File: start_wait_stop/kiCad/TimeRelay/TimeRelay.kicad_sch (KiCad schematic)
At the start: 15 parts, among them J1 230V AC Input, J10 Relay, J2 230V AC Input, J3 Relay, J4 Relay, J5 230V AC OUTPUT, J6 230V AC OUTPUT, J7 Relay, J8 Relay, J9 Relay, K1 FINDER-32.21-x000, SW1 Start

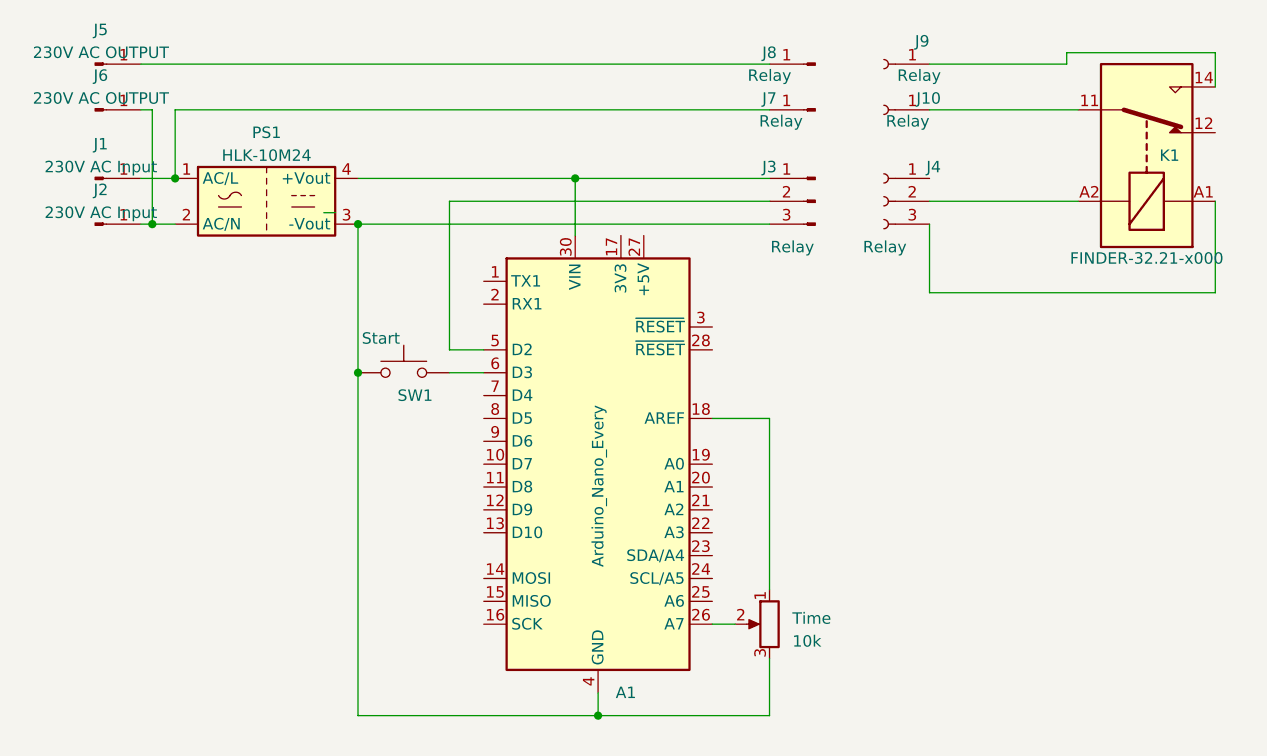
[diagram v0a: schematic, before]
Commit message: Playing arround witj KiCAD.
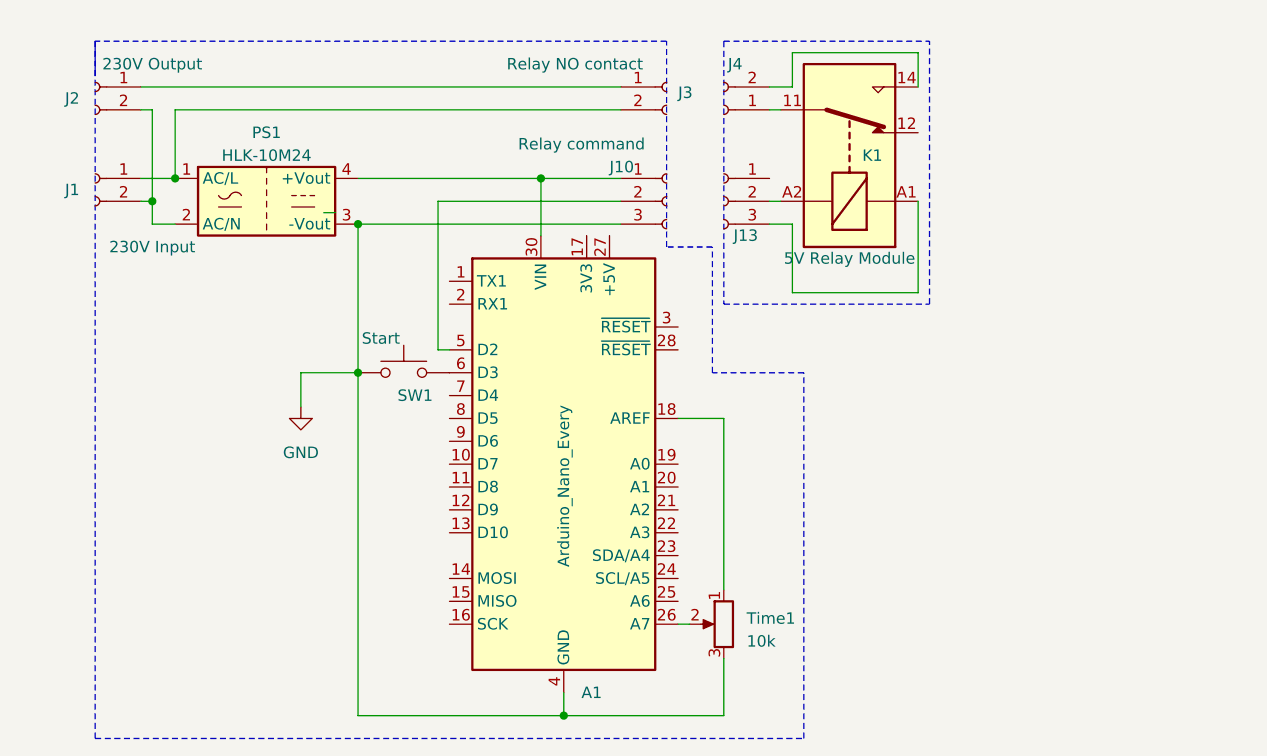
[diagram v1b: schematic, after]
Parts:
- removed J1, J2: 230V AC Input, symbol Connector:Conn_01x01_Pin
- removed J10, J9: Relay, symbol Connector:Conn_01x01_Socket
- removed J3: Relay, symbol Connector:Conn_01x03_Pin
- removed J4: Relay, symbol Connector:Conn_01x03_Socket
- removed J5, J6: 230V AC OUTPUT, symbol Connector:Conn_01x01_Pin
- removed J7, J8: Relay, symbol Connector:Conn_01x01_Pin
- added J1: 230V Input, Connector_Wire:SolderWire-1.5sqmm_1x02_P7.8mm_D1.7mm_OD3.9mm, symbol Connector:Conn_01x02_Socket
- added J10: Relay command, Connector_PinSocket_2.54mm:PinSocket_1x03_P2.54mm_Vertical, symbol Connector:Conn_01x03_Socket
- added J13: Relay, Connector_PinSocket_2.54mm:PinSocket_1x03_P2.54mm_Vertical, symbol Connector:Conn_01x03_Socket
- added J2: 230V Output, Connector_Wire:SolderWire-1.5sqmm_1x02_P7.8mm_D1.7mm_OD3.9mm, symbol Connector:Conn_01x02_Socket
- added J3: Relay NO contact, Connector_Wire:SolderWire-1.5sqmm_1x02_P7.8mm_D1.7mm_OD3.9mm, symbol Connector:Conn_01x02_Socket
- added J4: Conn_01x02_Socket, Connector_Wire:SolderWire-1.5sqmm_1x02_P7.8mm_D1.7mm_OD3.9mm, symbol Connector:Conn_01x02_Socket
- K1: value FINDER-32.21-x000 -> 5V Relay Module
- SW1: footprint (none) -> Button_Switch_THT:SW_Tactile_SPST_Angled_PTS645Vx83-2LFS
- Time1: renamed from Time; footprint (none) -> Potentiometer_THT:Potentiometer_Alps_RK09L_Single_Vertical
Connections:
- net at K1.14: now also J4.2 (Pin_2)
- net at PS1.1 (AC/L): now also J1.1 (Pin_1), J3.2 (Pin_2)
- net at PS1.2 (AC/N): now also J1.2 (Pin_2), J2.2 (Pin_2)
- net GND: now reaches A1.29 (GND), A1.4 (GND), PS1.3 (-Vout), SW1.1, Time1.3
- net GND: now also J10.3 (Pin_3)
- net at A1.30 (VIN), PS1.4 (+Vout): now also J10.1 (Pin_1)
- net at A1.5 (D2): now also J10.2 (Pin_2)
- net at K1.A2: now also J13.2 (Pin_2)
- net at K1.A1: now also J13.3 (Pin_3)
- net at K1.11: now also J4.1 (Pin_1)
- new net: J2.1 (Pin_1), J3.1 (Pin_1)
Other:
- moved on the sheet: A1, K1, Time1
